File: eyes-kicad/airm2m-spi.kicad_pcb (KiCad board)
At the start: 2 copper layers, 111.5 x 89 mm, 3 parts, among them J1 Conn_01x16, J2 Conn_01x16, J3 Conn_01x08

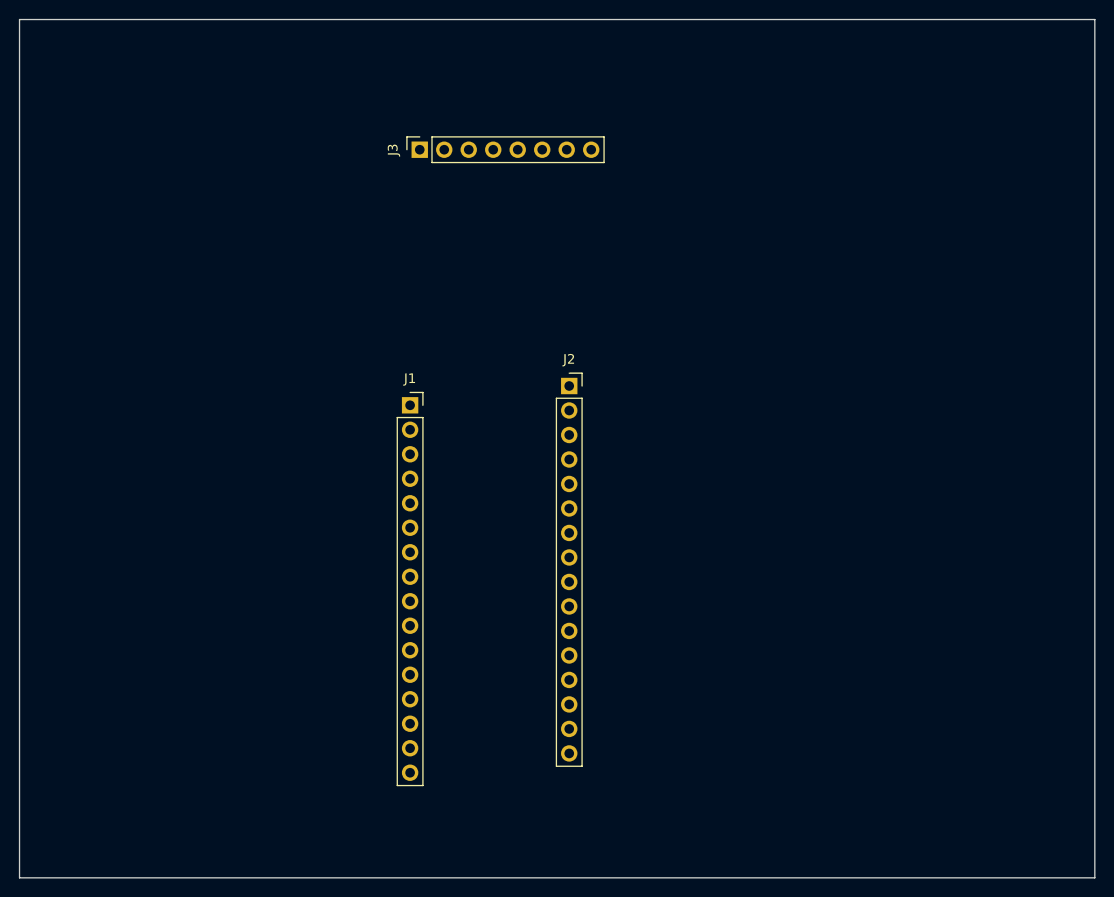
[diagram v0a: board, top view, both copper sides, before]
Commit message: chore: kicad
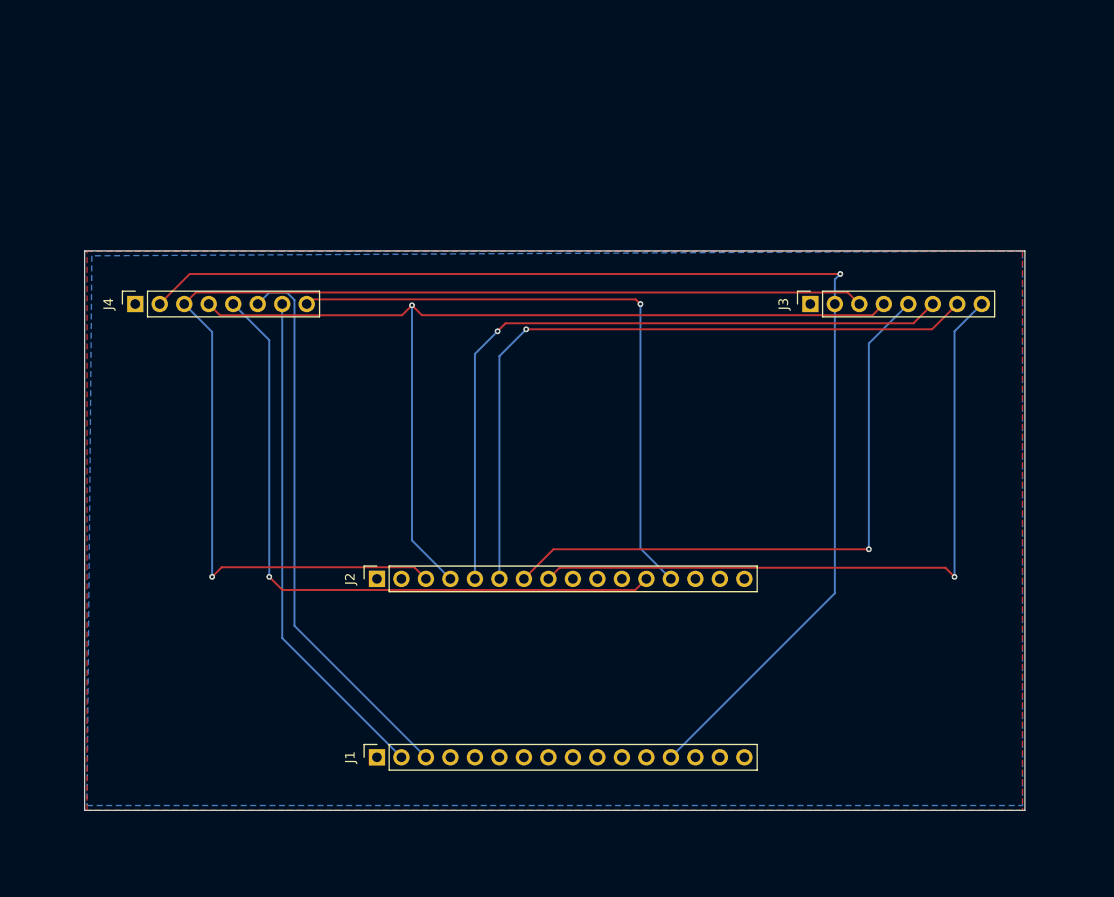
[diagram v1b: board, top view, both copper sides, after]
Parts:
- added J4: Conn_01x08, Connector_PinSocket_2.54mm:PinSocket_1x08_P2.54mm_Vertical, F.Cu at (71.5, 89.5)
- moved J3 43.5 mm to (141.5, 89.5)
- moved J1 36.7 mm to (96.6, 136.5), turned to 90 degrees
- moved J2 28.2 mm to (96.6, 118.0), turned to 90 degrees
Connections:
- J1 pad 2: (no net) -> N$7
- J1 pad 3: (no net) -> N$6
- J2 pad 12: (no net) -> N$5
- J2 pad 13: (no net) -> N$8
- J2 pad 3: N$1 (its old number) -> SPI_SCLK
- J2 pad 4: N$2 (its old number) -> SPI_MOSI
- J3 pad 3: N$1 (its old number) -> SPI_SCLK
- J3 pad 4: N$2 (its old number) -> SPI_MOSI
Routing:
- net 3V3: track 0.00 -> 132.5 mm, vias 0 -> 1
- net SPI_SCLK: track 0.00 -> 123.6 mm, vias 0 -> 1
- net SPI_MOSI: track 0.00 -> 101.8 mm, vias 0 -> 1
- net N$2: track 0.00 -> 72.9 mm, vias 0 -> 1
- net N$3: track 0.00 -> 72.8 mm, vias 0 -> 1
- net N$4: track 0.00 -> 72.4 mm, vias 0 -> 1
- net N$5: track 0.00 -> 70.0 mm, vias 0 -> 1
- net N$8: track 0.00 -> 64.8 mm, vias 0 -> 1
- net N$1: track 0.00 -> 64.2 mm, vias 0 -> 1
- net N$6: track 0.00 -> 57.7 mm
- net N$7: track 0.00 -> 52.1 mm
- added copper zone on B.Cu, net GND
- added copper zone on F.Cu, net GND
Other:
- board size 111.5 x 89 mm -> 97.5 x 58 mm
